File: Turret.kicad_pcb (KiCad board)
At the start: 2 copper layers, 104 x 54 mm, 27 parts, among them J1 172298-1108

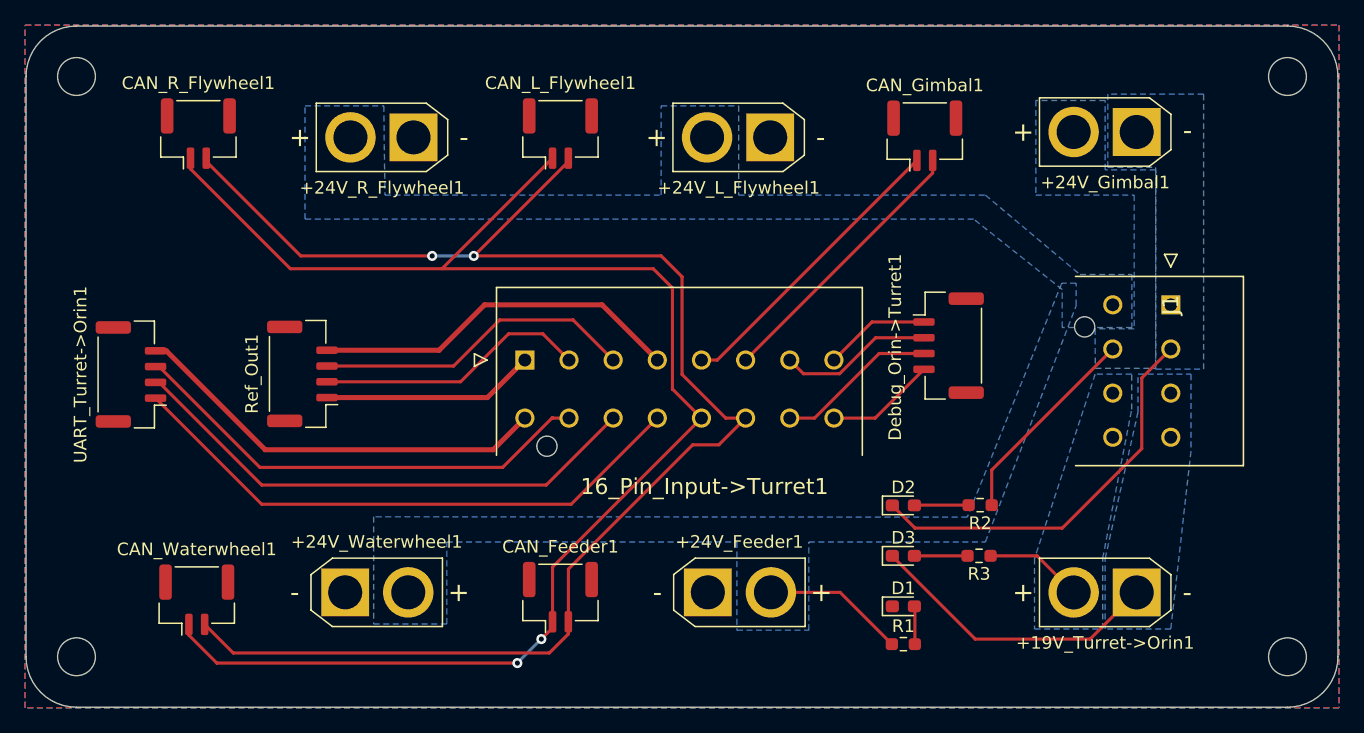
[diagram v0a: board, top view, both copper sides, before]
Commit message: Updated fab files
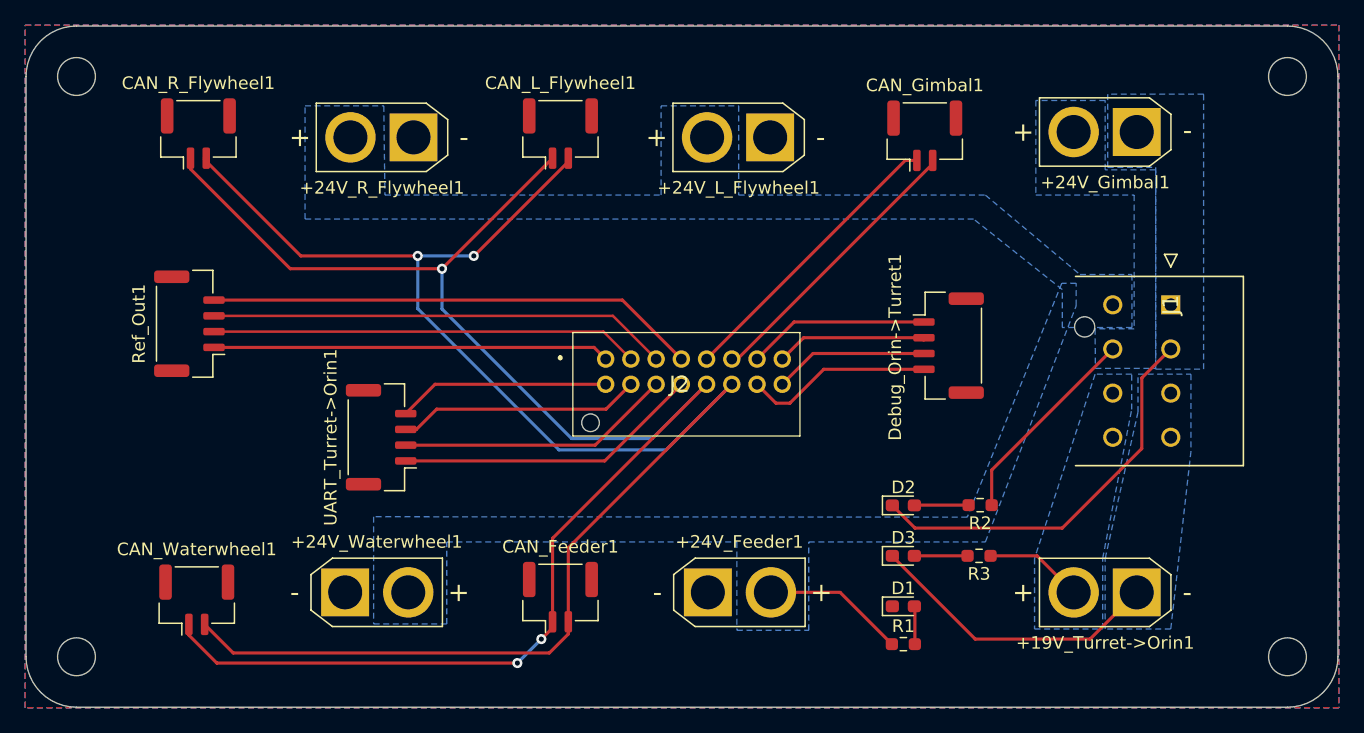
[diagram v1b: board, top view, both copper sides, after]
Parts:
- removed 16_Pin_Input->Turret1: 172298-1116, Connectors:172298-YY16
- removed G***: LOGO, LOGO
- added J2: 501645-1620, Connectors:5016451620, F.Cu at (92.2, 62.5)
- moved UART_Turret->Orin1 20.4 mm to (68.6, 66.7)
- moved Ref_Out1 9.80 mm to (53.4, 57.7)
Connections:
- Ref_Out1 pad 2: /Ref_CANL -> /Ref_CAN-
- Ref_Out1 pad 3: /Ref_CANH -> /Ref_CAN+
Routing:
- net /Ref_CAN+: track 0.00 -> 36.5 mm
- net /Ref_CAN-: track 0.00 -> 34.0 mm
- net /Ref_CANH: track 25.5 -> 0.00 mm
- net /UART_GND: track 46.1 -> 24.4 mm
- net /Ref_CANL: track 21.6 -> 0.00 mm
- net /UART_TX: track 41.8 -> 21.8 mm
- net /UART_RX: track 37.7 -> 19.3 mm
- net /UART_3V3: track 33.6 -> 16.8 mm
- net /Ref_GND: track 16.9 -> 31.4 mm
- net /Ref_PWR: track 29.5 -> 39.0 mm
- net /SWD_3V3: track 8.74 -> 15.0 mm
- net /SWD_GND: track 8.39 -> 14.5 mm
- net /CANH: track 122.0 -> 127.2 mm
- net /CANL: track 120.4 -> 123.3 mm, vias 2 -> 3
- net /CANGim_H: track 22.0 -> 22.6 mm
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
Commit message: Updated fab files
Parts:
- J1: footprint Connectors:172298-YY08 -> Robomaster_Connectors:172298-YY08
- J2: footprint Connectors:5016451620 -> Robomaster_Connectors:5016451620
